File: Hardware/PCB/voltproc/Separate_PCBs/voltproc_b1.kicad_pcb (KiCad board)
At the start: 2 copper layers, 71 x 174 mm, 77 parts, among them J1 Synth_power_2x5, J10 Jack, J11 Jack, J12 Jack, J13 Jack, J14 Jack, J15 Jack, J16 Jack, J17 Jack, J18 Jack, J19 Jack, J2 3_pin_Molex_header, J3 3_pin_Molex_header, J4 Conn_01x13, J8 Jack, J9 Jack, U1 TL074, U2 TL074, U3 TL072

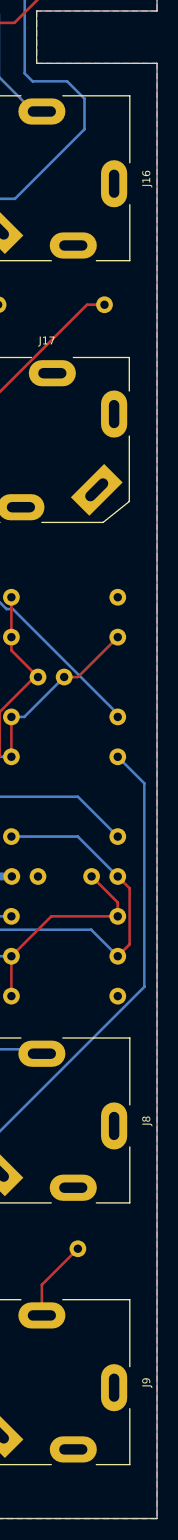
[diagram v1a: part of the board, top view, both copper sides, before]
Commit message: gerbers
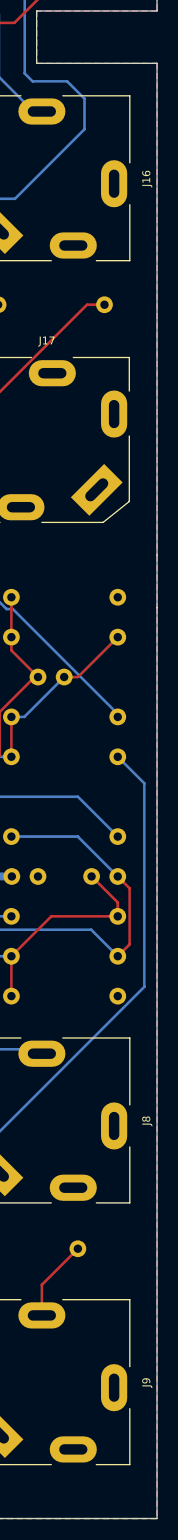
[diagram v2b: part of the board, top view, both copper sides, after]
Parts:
- added B1: Board, ao_tht:Board_Marker, F.Cu at (48.5, 15.0)
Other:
- outline, holes or cut-outs redrawn
